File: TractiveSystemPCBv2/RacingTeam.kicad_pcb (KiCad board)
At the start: 4 copper layers, 122.5 x 92.5 mm, 93 parts, among them J1 BusIn, J10 BatteryIn, J11 ShutdownIn, J2 Bypass Pin, J3 BypassPin, J4 BypassPin, J5 BypassPin, J6 PC Relay, J7 AIROut, J8 Discharge Relay Out, J9 Molex, Q1 TP0610T, Q2 2N7002, Q3 2N7002, Q4 TP0610T, Q5 2N7002, Q6 TP0610T, Q7 2N7002, Q8 TP0610T, Q9 TP0610T, U1 LM311, U2 LM311, U3 4N35, U4 MC78M12ABDTRKG, U6 NE555D

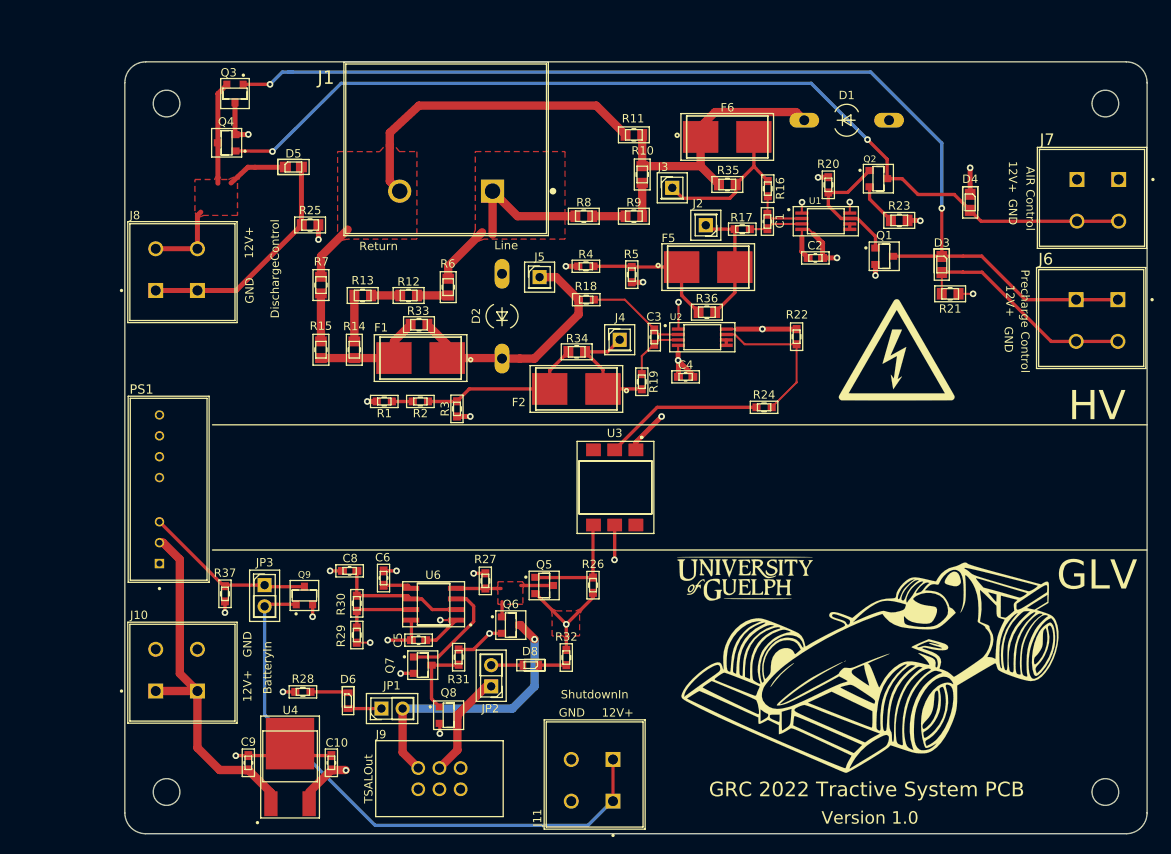
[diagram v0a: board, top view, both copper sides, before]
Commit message: Update RacingTeam.kicad_pcb-bak, RacingTeam.xml, and 38 more files...
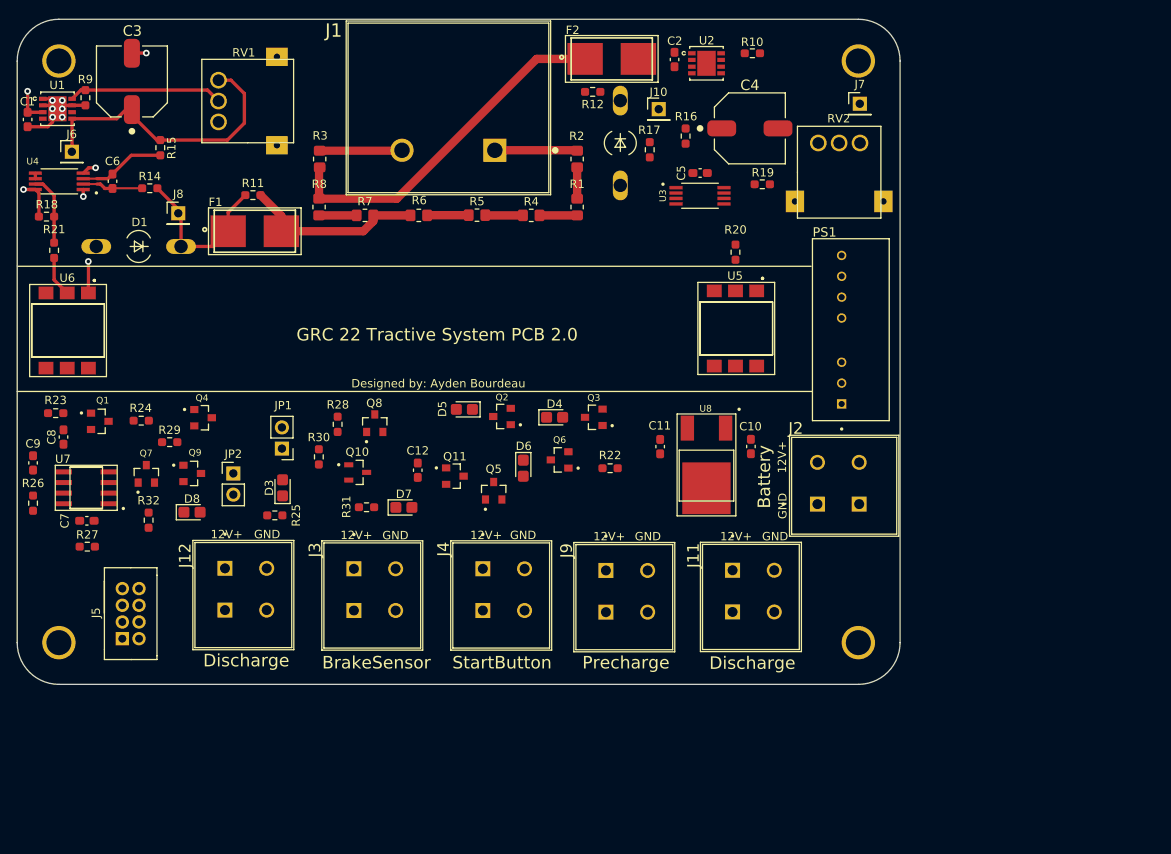
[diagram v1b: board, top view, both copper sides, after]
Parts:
- removed F5, F6: Fuse_Small, GRC22Footprints:FUSE_0154004.DRTL
- removed G***: LOGO, Footprints:PCB
- removed G***: LOGO, Footprints:UofGLogo
- removed G***: LOGO, Footprints:HVLogo
- removed JP3: Jumper, GRC22Footprints:PinHeader_1x02_P2.54mm_Vertical
- removed R13: 249kΩ, GRC22Footprints:R_0805_2012Metric_Pad1.20x1.40mm_HandSolder
- removed R33, R34, R35, R36: 0Ω, GRC22Footprints:R_0805_2012Metric_Pad1.20x1.40mm_HandSolder
- removed R37: 4kΩ, GRC22Footprints:R_0603_1608Metric_Pad0.98x0.95mm_HandSolder
- removed the REF** at (114.5, 118.5)
- removed the REF** at (114.5, 36.0)
- removed the REF** at (227.0, 36.0)
- removed the REF** at (227.0, 118.5)
- added C11: 1μF, TractiveSystemLib:C_0603_1608Metric_Pad1.08x0.95mm_HandSolder, F.Cu at (173.7, 77.1)
- added C12: 1μF, TractiveSystemLib:C_0603_1608Metric_Pad1.08x0.95mm_HandSolder, F.Cu at (144.6, 79.9)
- added C7: 100nF, TractiveSystemLib:C_0603_1608Metric_Pad1.08x0.95mm_HandSolder, F.Cu at (105.0, 86.0)
- added D7: D, TractiveSystemLib:D_0805_2012Metric_Castellated, F.Cu at (142.9, 84.4)
- added J12: DischargeRelay, TractiveSystemLib:CUI_TBL001-500-02GY-2GY, F.Cu at (121.5, 91.7)
- added Q10: Q_NPN_BCE, TractiveSystemLib:SOT91P240X110-3N, F.Cu at (137.4, 80.2)
- added Q11: RSC, TractiveSystemLib:BZT03C12-TR, F.Cu at (149.1, 80.7)
- added REF**: 2-56Mount, TractiveSystemLib:2-56Mount, F.Cu at (197.4, 30.9)
- added REF**: 2-56Mount, TractiveSystemLib:2-56Mount, F.Cu at (101.6, 100.6)
- added REF**: 2-56Mount, TractiveSystemLib:2-56Mount, F.Cu at (197.4, 100.6)
- added REF**: 2-56Mount, TractiveSystemLib:2-56Mount, F.Cu at (101.6, 30.9)
- added RV1: 10kΩ, TractiveSystemLib:PT01-D120K2-B103, F.Cu at (124.2, 35.7)
- added RV2: 10kΩ, TractiveSystemLib:PT01-D120K2-B103, F.Cu at (195.1, 44.2)
- added U5: 4N35, TractiveSystemLib:OPTO_4N35SM, F.Cu at (182.7, 63.0)
- added U7: NE555D, TractiveSystemLib:NE555PSRE4, F.Cu at (104.9, 82.0)
- added U8: MC78M12ABDTRKG, TractiveSystemLib:TO229P990X238-4N, F.Cu at (179.2, 79.6)
- C1: value 10nF -> 470nF; footprint GRC22Footprints:C_0603_1608Metric_Pad1.08x0.95mm_HandSolder -> TractiveSystemLib:C_0603_1608Metric_Pad1.08x0.95mm_HandSolder
- C10, C9: footprint GRC22Footprints:C_0603_1608Metric_Pad1.08x0.95mm_HandSolder -> TractiveSystemLib:C_0603_1608Metric_Pad1.08x0.95mm_HandSolder
- C2: value 0.1uF -> 470nF; footprint GRC22Footprints:C_0603_1608Metric_Pad1.08x0.95mm_HandSolder -> TractiveSystemLib:C_0603_1608Metric_Pad1.08x0.95mm_HandSolder
- C3: value 10nF -> 22μF; footprint GRC22Footprints:C_0603_1608Metric_Pad1.08x0.95mm_HandSolder -> TractiveSystemLib:CAPE830X690N
- C4: value 0.1uF -> 22μF; footprint GRC22Footprints:C_0603_1608Metric_Pad1.08x0.95mm_HandSolder -> TractiveSystemLib:CAPE830X690N
- C5, C6: value 100nF -> 10nF; footprint GRC22Footprints:C_0603_1608Metric_Pad1.08x0.95mm_HandSolder -> TractiveSystemLib:C_0603_1608Metric_Pad1.08x0.95mm_HandSolder
- C8: value 1μF -> 100nF; footprint GRC22Footprints:C_0603_1608Metric_Pad1.08x0.95mm_HandSolder -> TractiveSystemLib:C_0603_1608Metric_Pad1.08x0.95mm_HandSolder
- D1, D2: footprint GRC22Footprints:SOD57-10 -> TractiveSystemLib:SOD57-10
- D3: value Flyback -> LED; footprint GRC22Footprints:D_0805_2012Metric_Castellated -> TractiveSystemLib:D_0805_2012Metric_Castellated
- D4, D5: footprint GRC22Footprints:D_0805_2012Metric_Castellated -> TractiveSystemLib:D_0805_2012Metric_Castellated
- D6: value LED -> Flyback; footprint GRC22Footprints:D_0603_1608Metric_Castellated -> TractiveSystemLib:D_0805_2012Metric_Castellated
- D8: footprint GRC22Footprints:D_0603_1608Metric_Castellated -> TractiveSystemLib:D_0805_2012Metric_Castellated
- F1, F2: footprint GRC22Footprints:FUSE_0154004.DRTL -> TractiveSystemLib:FUSE_0154004.DRTL
- J1: footprint GRC22Footprints:TE_8PCV-02-006 -> TractiveSystemLib:TE_8PCV-02-006
- J10: value BatteryIn -> BypassPin; footprint GRC22Footprints:CUI_TBL001-500-02GY-2GY -> TractiveSystemLib:PinHeader_1x01_P2.54mm_Vertical
- J11: value ShutdownIn -> AIR Out; footprint GRC22Footprints:CUI_TBL001-500-02GY-2GY -> TractiveSystemLib:CUI_TBL001-500-02GY-2GY
- J2: value Bypass Pin -> PowerInput; footprint GRC22Footprints:PinHeader_1x01_P2.54mm_Vertical -> TractiveSystemLib:CUI_TBL001-500-02GY-2GY
- J3: value BypassPin -> BrakePositionSensor; footprint GRC22Footprints:PinHeader_1x01_P2.54mm_Vertical -> TractiveSystemLib:CUI_TBL001-500-02GY-2GY
- J4: value BypassPin -> StartButton; footprint GRC22Footprints:PinHeader_1x01_P2.54mm_Vertical -> TractiveSystemLib:CUI_TBL001-500-02GY-2GY
- J5: value BypassPin -> Molex; footprint GRC22Footprints:PinHeader_1x01_P2.54mm_Vertical -> TractiveSystemLib:878310819
- J6: value PC Relay -> BypassPin; footprint GRC22Footprints:CUI_TBL001-500-02GY-2GY -> TractiveSystemLib:PinHeader_1x01_P2.54mm_Vertical
- J7: value AIROut -> Bypass Pin; footprint GRC22Footprints:CUI_TBL001-500-02GY-2GY -> TractiveSystemLib:PinHeader_1x01_P2.54mm_Vertical
- J8: value Discharge Relay Out -> BypassPin; footprint GRC22Footprints:CUI_TBL001-500-02GY-2GY -> TractiveSystemLib:PinHeader_1x01_P2.54mm_Vertical
- J9: value Molex -> PC Out; footprint GRC22Footprints:Molex -> TractiveSystemLib:CUI_TBL001-500-02GY-2GY
- JP1, JP2: footprint GRC22Footprints:PinHeader_1x02_P2.54mm_Vertical -> TractiveSystemLib:PinHeader_1x02_P2.54mm_Vertical
- PS1: footprint GRC22Footprints:CONV_SPBW06F-12 -> TractiveSystemLib:CONV_SPBW06F-12
- Q1: value TP0610T -> 2N7002; footprint GRC22Footprints:2N7002H6327XTSA2_v2 -> TractiveSystemLib:2N7002H6327XTSA2
- Q2, Q3, Q7: footprint GRC22Footprints:2N7002H6327XTSA2 -> TractiveSystemLib:2N7002H6327XTSA2
- Q4, Q8, Q9: footprint GRC22Footprints:2N7002H6327XTSA2_v2 -> TractiveSystemLib:BZT03C12-TR
- Q5: value 2N7002 -> TP0610T; footprint GRC22Footprints:2N7002H6327XTSA2 -> TractiveSystemLib:BZT03C12-TR
- Q6: value TP0610T -> RSC; footprint GRC22Footprints:2N7002H6327XTSA2_v2 -> TractiveSystemLib:BZT03C12-TR
- R1, R2: value 1.3kΩ -> 200kΩ; footprint GRC22Footprints:R_0603_1608Metric_Pad0.98x0.95mm_HandSolder -> TractiveSystemLib:R_0805_2012Metric_Pad1.20x1.40mm_HandSolder
- R10, R9: value 150kΩ -> 1kΩ; footprint GRC22Footprints:R_0805_2012Metric_Pad1.20x1.40mm_HandSolder -> TractiveSystemLib:R_0603_1608Metric_Pad0.98x0.95mm_HandSolder
- R11: value 4kΩ -> 0Ω; footprint GRC22Footprints:R_0805_2012Metric_Pad1.20x1.40mm_HandSolder -> TractiveSystemLib:R_0603_1608Metric_Pad0.98x0.95mm_HandSolder
- R12: value 249kΩ -> 0Ω; footprint GRC22Footprints:R_0805_2012Metric_Pad1.20x1.40mm_HandSolder -> TractiveSystemLib:R_0603_1608Metric_Pad0.98x0.95mm_HandSolder
- R14: value 249kΩ -> 100Ω; footprint GRC22Footprints:R_0805_2012Metric_Pad1.20x1.40mm_HandSolder -> TractiveSystemLib:R_0603_1608Metric_Pad0.98x0.95mm_HandSolder
- R15: value 49kΩ -> 100Ω; footprint GRC22Footprints:R_0805_2012Metric_Pad1.20x1.40mm_HandSolder -> TractiveSystemLib:R_0603_1608Metric_Pad0.98x0.95mm_HandSolder
- R16, R17, R32: footprint GRC22Footprints:R_0603_1608Metric_Pad0.98x0.95mm_HandSolder -> TractiveSystemLib:R_0603_1608Metric_Pad0.98x0.95mm_HandSolder
- R18, R19: value 100Ω -> 20kΩ; footprint GRC22Footprints:R_0603_1608Metric_Pad0.98x0.95mm_HandSolder -> TractiveSystemLib:R_0603_1608Metric_Pad0.98x0.95mm_HandSolder
- R20: value 20kΩ -> 1.2kΩ; footprint GRC22Footprints:R_0603_1608Metric_Pad0.98x0.95mm_HandSolder -> TractiveSystemLib:R_0603_1608Metric_Pad0.98x0.95mm_HandSolder
- R21: value 0Ω -> 1.2kΩ; footprint GRC22Footprints:R_0805_2012Metric_Pad1.20x1.40mm_HandSolder -> TractiveSystemLib:R_0603_1608Metric_Pad0.98x0.95mm_HandSolder
- R22: value 20kΩ -> 10kΩ; footprint GRC22Footprints:R_0603_1608Metric_Pad0.98x0.95mm_HandSolder -> TractiveSystemLib:R_0603_1608Metric_Pad0.98x0.95mm_HandSolder
- R23: value 0Ω -> 10kΩ; footprint GRC22Footprints:R_0805_2012Metric_Pad1.20x1.40mm_HandSolder -> TractiveSystemLib:R_0603_1608Metric_Pad0.98x0.95mm_HandSolder
- R24: value 1.2kΩ -> 22kΩ; footprint GRC22Footprints:R_0603_1608Metric_Pad0.98x0.95mm_HandSolder -> TractiveSystemLib:R_0603_1608Metric_Pad0.98x0.95mm_HandSolder
- R25: value 0Ω -> 499Ω; footprint GRC22Footprints:R_0805_2012Metric_Pad1.20x1.40mm_HandSolder -> TractiveSystemLib:R_0603_1608Metric_Pad0.98x0.95mm_HandSolder
- R26: value 10kΩ -> 22kΩ; footprint GRC22Footprints:R_0603_1608Metric_Pad0.98x0.95mm_HandSolder -> TractiveSystemLib:R_0603_1608Metric_Pad0.98x0.95mm_HandSolder
- R27: value 22kΩ -> 220kΩ; footprint GRC22Footprints:R_0603_1608Metric_Pad0.98x0.95mm_HandSolder -> TractiveSystemLib:R_0603_1608Metric_Pad0.98x0.95mm_HandSolder
- R28: value 499Ω -> 10kΩ; footprint GRC22Footprints:R_0603_1608Metric_Pad0.98x0.95mm_HandSolder -> TractiveSystemLib:R_0603_1608Metric_Pad0.98x0.95mm_HandSolder
- R29: value 22kΩ -> 10kΩ; footprint GRC22Footprints:R_0603_1608Metric_Pad0.98x0.95mm_HandSolder -> TractiveSystemLib:R_0603_1608Metric_Pad0.98x0.95mm_HandSolder
- R3: value 1.3kΩ -> 25kΩ; footprint GRC22Footprints:R_0603_1608Metric_Pad0.98x0.95mm_HandSolder -> TractiveSystemLib:R_0805_2012Metric_Pad1.20x1.40mm_HandSolder
- R30: value 220kΩ -> 47kΩ; footprint GRC22Footprints:R_0603_1608Metric_Pad0.98x0.95mm_HandSolder -> TractiveSystemLib:R_0603_1608Metric_Pad0.98x0.95mm_HandSolder
- R31: value 10kΩ -> 4.7kΩ; footprint GRC22Footprints:R_0603_1608Metric_Pad0.98x0.95mm_HandSolder -> TractiveSystemLib:R_0603_1608Metric_Pad0.98x0.95mm_HandSolder
- R4: value 4.7kΩ -> 500kΩ; footprint GRC22Footprints:R_0603_1608Metric_Pad0.98x0.95mm_HandSolder -> TractiveSystemLib:R_0805_2012Metric_Pad1.20x1.40mm_HandSolder
- R5: value 6.8kΩ -> 500kΩ; footprint GRC22Footprints:R_0603_1608Metric_Pad0.98x0.95mm_HandSolder -> TractiveSystemLib:R_0805_2012Metric_Pad1.20x1.40mm_HandSolder
- R6: value 249kΩ -> 150kΩ; footprint GRC22Footprints:R_0805_2012Metric_Pad1.20x1.40mm_HandSolder -> TractiveSystemLib:R_0805_2012Metric_Pad1.20x1.40mm_HandSolder
- R7: value 22kΩ -> 150kΩ; footprint GRC22Footprints:R_0805_2012Metric_Pad1.20x1.40mm_HandSolder -> TractiveSystemLib:R_0805_2012Metric_Pad1.20x1.40mm_HandSolder
- R8: value 150kΩ -> 25kΩ; footprint GRC22Footprints:R_0805_2012Metric_Pad1.20x1.40mm_HandSolder -> TractiveSystemLib:R_0805_2012Metric_Pad1.20x1.40mm_HandSolder
- U1, U2: value LM311 -> LM2941LD; footprint GRC22Footprints:LM311PW -> TractiveSystemLib:DFN400X400X80-9N
- U3: value 4N35 -> LM311; footprint GRC22Footprints:OPTO_4N35SM -> TractiveSystemLib:LM311PW
- U4: value MC78M12ABDTRKG -> LM311; footprint GRC22Footprints:TO229P990X238-4N -> TractiveSystemLib:LM311PW
- U6: value NE555D -> 4N35; footprint GRC22Footprints:NE555PSRE4 -> TractiveSystemLib:OPTO_4N35SM
- moved J6 126.6 mm to (103.2, 41.8), turned to 0 degrees
- moved R21 107.5 mm to (101.0, 53.6), turned to 270 degrees
- moved R23 103.7 mm to (101.2, 73.1)
- moved Q1 96.1 mm to (106.5, 74.1)
- moved U1 93.1 mm to (101.4, 36.6)
- moved J10 92.2 mm to (173.5, 36.7), turned to 0 degrees
- moved C1 89.5 mm to (97.8, 37.9)
- moved D1 86.2 mm to (111.2, 53.1), turned to 180 degrees
- moved PS1 84.0 mm to (196.5, 63.1)
- moved D3 83.4 mm to (128.4, 82.0), turned to 90 degrees
- moved U4 75.2 mm to (101.7, 45.3), turned to 180 degrees
- moved R24 74.7 mm to (111.5, 74.0)
- moved C3 69.7 mm to (110.3, 33.4), turned to 90 degrees
- moved R26 67.8 mm to (98.5, 83.9), turned to 90 degrees
- moved R9 67.2 mm to (104.8, 35.3), turned to 90 degrees
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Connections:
- C1 pad 1: /PreChargeV+ -> +12V
- C1 pad 2: /PrechargeV- -> GND
- C10 pad 1: GLV+ -> +BATT
- C2 pad 1: GND -> +12V
- C3 pad 1: /TSAL_LM311V+ -> /TSALRef
- C3 pad 2: /TSAL_LM311V- -> GND
- C4 pad 1: GND -> /PrechargeRef
- C5 pad 1: GLV+ -> /PreChargeV+
- C5 pad 2: GLV- -> /PrechargeV-
- C6 pad 1: Net-(C6-Pad1) -> /TSAL_LM311V+
- C6 pad 2: GLV- -> /TSAL_LM311V-
- C8 pad 1: /555Trigger -> Net-(C8-Pad1)
- C9 pad 1: +BATT -> /555Trigger
- D1 pad 1: /PrechargeBus -> /BusRefTSAL
- D2 pad 1: /BusRefTSAL -> Net-(D2-Pad1)
- D3 pad 1: /PreChargeON -> /OBLEDResistorGreen
- D3 pad 2: /PrechargeRelayOut -> /OBLEDGreen
- D4 pad 1: +12V -> GLV+
- D4 pad 2: /AIRON -> /Precharge-
- D5 pad 1: /DischargeIn -> /Discharge
- D5 pad 2: /DischargeOut -> GLV-
- D6 pad 1: /OBLEDResistorGreen -> /AIR+
- D6 pad 2: /OBLEDGreen -> GLV-
- F2 pad 1: /TSALRef -> /BusOutPrecharge
- F2 pad 2: /TSALREFOut -> Net-(D2-Pad1)
- J10 pad 1: +BATT -> Net-(D2-Pad1)
- J11 pad 1: /Shutdown -> /AIR+
- J2 pad 1: /PrechargeTP- -> GLV-
- J3 pad 1: /PrechargeTP+ -> /RTDLatch
- J4 pad 1: /TSALRef -> /Common
- J5 pad 1: /BusRefTSAL -> GLV+
- J6 pad 1: /PreChargeON -> /TSALRef
- J7 pad 1: +12V -> /PrechargeRef
- J8 pad 1: /DischargeOut -> /BusRefTSAL
- J9 pad 2: /Green+ -> /Precharge-
- PS1 pad 3: /Enable -> Net-(PS1-Pad3)
- Q1 pad 1: /PrechargeCompOUT -> /InvertBus
- Q1 pad 2: +12V -> GLV-
- Q1 pad 3: /PreChargeON -> /555Reset
- Q2 pad 1: /PrechargeCompOUT -> /AIR+
- Q2 pad 2: Net-(Q2-Pad2) -> /Discharge
- Q2 pad 3: /AIRON -> GLV+
- Q3 pad 1: /PreChargeON -> /PrechargeOPTO
- Q3 pad 2: /DischargeIn -> GLV-
- Q3 pad 3: +12V -> /Precharge-
- Q4 pad 1: /AIRON -> /555Reset
- Q4 pad 2: +12V -> GLV+
- Q4 pad 3: /DischargeIn -> /Green+
- Q5 pad 1: /InvertBus -> /Precharge-
- Q5 pad 2: GLV- -> GLV+
- Q5 pad 3: /555Reset -> /Discharge
- Q6 pad 1: /555Reset -> /PrechargeOPTO
- Q6 pad 3: /Green+ -> /AIR+
- Q8 pad 1: /555DriveRED -> /RTDLatch
- Q8 pad 3: /RED+ -> /RTDOutput
- Q9 pad 1: /Shutdown -> /555DriveRED
- Q9 pad 3: /Enable -> /RED+
- R1 pad 2: +12V -> Net-(R1-Pad2)
- R10 pad 1: Net-(R10-Pad1) -> GND
- R10 pad 2: /PrechargeBus -> Net-(R10-Pad2)
- R11 pad 1: /PrechargeBus -> /BusRefTSAL
- R11 pad 2: /BusReturn -> /BusOutTSAL
- R12 pad 1: Net-(R12-Pad1) -> Net-(D2-Pad1)
- R12 pad 2: Net-(R12-Pad2) -> /BusOutPrecharge
- R14 pad 1: Net-(R13-Pad2) -> /TSAL_LM311V+
- R14 pad 2: /BusOutTSAL -> /BusRefTSAL
- R15 pad 1: /BusOutTSAL -> /TSAL_LM311V-
- R15 pad 2: Net-(R15-Pad2) -> /TSALRef
- R16 pad 1: /PreChargeV+ -> /PrechargeV-
- R16 pad 2: /PrechargeTP+ -> /PrechargeRef
- R17 pad 1: /PrechargeV- -> /PreChargeV+
- R17 pad 2: /PrechargeTP- -> Net-(D2-Pad1)
- R18 pad 1: /TSAL_LM311V+ -> /TSALCompOut
- R18 pad 2: /BusRefTSAL -> +12V
- R19 pad 1: /TSAL_LM311V- -> /PrechargeCompOUT
- R19 pad 2: /TSALRef -> +12V
- R2 pad 1: /TSALREFOut -> /BusLine
- R20 pad 2: +12V -> Net-(R20-Pad2)
- R21 pad 1: GND -> /TSALCompOut
- R21 pad 2: /PrechargeRelayOut -> Net-(R21-Pad2)
- R22 pad 1: /TSALCompOut -> GLV-
- R22 pad 2: +12V -> /PrechargeOPTO
- R23 pad 1: GND -> /InvertBus
- R23 pad 2: Net-(Q2-Pad2) -> GLV-
- R24 pad 1: /TSALCompOut -> GLV+
- R24 pad 2: Net-(R24-Pad2) -> /555Reset
- R25 pad 1: GND -> /OBLEDResistorGreen
- R25 pad 2: /DischargeOut -> GLV-
- R26 pad 1: /InvertBus -> GLV+
- R26 pad 2: GLV- -> /555Discharge
- R27 pad 1: GLV+ -> /555Discharge
- R27 pad 2: /555Reset -> /555Trigger
- R28 pad 1: /OBLEDResistorGreen -> /RTDLatch
- R28 pad 2: GLV- -> GLV+
- R29 pad 2: /555Discharge -> /555DriveRED
- R3 pad 1: GND -> /BusOutPrecharge
- R3 pad 2: /TSALREFOut -> /BusReturn
- R30 pad 1: /555Discharge -> Net-(Q10-Pad1)
- R30 pad 2: /555Trigger -> GLV-
- R31 pad 1: GLV+ -> Net-(Q10-Pad1)
- R31 pad 2: /555DriveRED -> Net-(C12-Pad2)
- R4 pad 1: +12V -> Net-(R4-Pad1)
- R4 pad 2: /PrechargeRef2 -> Net-(R1-Pad2)
- R5 pad 1: /PrechargeRef2 -> Net-(R5-Pad1)
- R5 pad 2: GND -> Net-(R4-Pad1)
- R6 pad 1: Net-(R12-Pad2) -> Net-(R5-Pad1)
- R6 pad 2: /BusLine -> /BusOutTSAL
- R7 pad 1: Net-(R15-Pad2) -> /BusOutTSAL
- R7 pad 2: /BusReturn -> Net-(R7-Pad2)
- R8 pad 1: /BusLine -> Net-(R7-Pad2)
- R8 pad 2: Net-(R8-Pad2) -> /BusOutPrecharge
- R9 pad 1: Net-(R8-Pad2) -> GND
- R9 pad 2: Net-(R10-Pad1) -> Net-(R9-Pad2)
- U1 pad 2: /PreChargeV+ -> GND
- U1 pad 3: /PrechargeV- -> +12V
- U1 pad 4: GND -> Net-(U1-Pad4)
- U1 pad 5: Net-(U1-Pad5) -> /TSALRef
- U1 pad 6: Net-(U1-Pad5) -> Net-(U1-Pad6)
- U1 pad 7: /PrechargeCompOUT -> GND
- U1 pad 8: +12V -> Net-(R9-Pad2)
- U2 pad 2: /TSAL_LM311V+ -> GND
- U2 pad 3: /TSAL_LM311V- -> +12V
- U2 pad 4: GND -> Net-(U2-Pad4)
- U2 pad 5: Net-(U2-Pad5) -> /PrechargeRef
- U2 pad 6: Net-(U2-Pad5) -> Net-(U2-Pad6)
- U2 pad 7: /TSALCompOut -> GND
- U2 pad 8: +12V -> Net-(R10-Pad2)
- U3 pad 1: +12V -> GND
- U3 pad 2: Net-(R24-Pad2) -> /PreChargeV+
- U3 pad 3: (no net) -> /PrechargeV-
- U3 pad 4: /InvertBus -> GND
- U3 pad 5: GLV+ -> Net-(U3-Pad5)
- U3 pad 6: Net-(U3-Pad6) -> Net-(U3-Pad5)
- U4 pad 1: +BATT -> GND
- U4 pad 3: GLV+ -> /TSAL_LM311V-
- U4 pad 4: GLV- -> GND
- U6 pad 1: GLV- -> +12V
- U6 pad 2: /555Trigger -> Net-(R21-Pad2)
- U6 pad 3: /555Output -> (no net)
- U6 pad 4: /555Reset -> /InvertBus
- U6 pad 5: Net-(C6-Pad1) -> GLV+
- U6 pad 6: /555Trigger -> Net-(U6-Pad6)
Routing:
- net /PreChargeON: track 130.9 -> 0.00 mm, vias 2 -> 0
- net /AIRON: track 117.4 -> 0.00 mm, vias 2 -> 0
- net /Shutdown: track 70.3 -> 0.00 mm
- net +BATT: track 44.1 -> 0.00 mm
- net /BusOutPrecharge: track 0.00 -> 42.6 mm
- net GLV-: track 41.9 -> 0.00 mm, vias 8 -> 0
- net /BusReturn: track 45.4 -> 9.88 mm
- net /Green+: track 33.0 -> 0.00 mm, vias 1 -> 0
- net /PrechargeBus: track 32.1 -> 0.00 mm
- net /DischargeIn: track 29.1 -> 0.00 mm
- net /DischargeOut: track 28.3 -> 0.00 mm
- net GLV+: track 28.1 -> 0.00 mm, vias 8 -> 0
- net /PrechargeRelayOut: track 27.1 -> 0.00 mm
- net /Enable: track 20.6 -> 0.00 mm
- net /TSALREFOut: track 20.1 -> 0.00 mm
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- added copper zone on PWR, net +BATT
- removed copper zone on F.Cu, net /555Reset
- removed copper zone on F.Cu, net /BusLine
- removed copper zone on F.Cu, net /BusReturn
- removed copper zone on F.Cu, net /DischargeIn
- removed copper zone on F.Cu, net GLV-
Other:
- board size 122.5 x 92.5 mm -> 105.8 x 79.7 mm
- board text added: "Battery"
- board text added: "BrakeSensor"
- board text added: "Designed by: Ayden Bourdeau"
- board text added: "Discharge"
- board text added: "GRC 22 Tractive System PCB 2.0"
- board text added: "Precharge"
- board text added: "StartButton"
- board text removed: "AIR Control"
- board text removed: "BatteryIn"
- board text removed: "DischargeControl"
- board text removed: "GLV"
- board text removed: "GRC 2022 Tractive System PCB"
- board text removed: "HV"
- board text removed: "Line"
- board text removed: "Precharge Control"
- board text removed: "Return"
- board text removed: "ShutdownIn"
- board text removed: "TSALOut"
- board text removed: "Version 1.0"
